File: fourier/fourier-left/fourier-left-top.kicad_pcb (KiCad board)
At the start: 2 copper layers, 136.6 x 96.2 mm, 7 parts

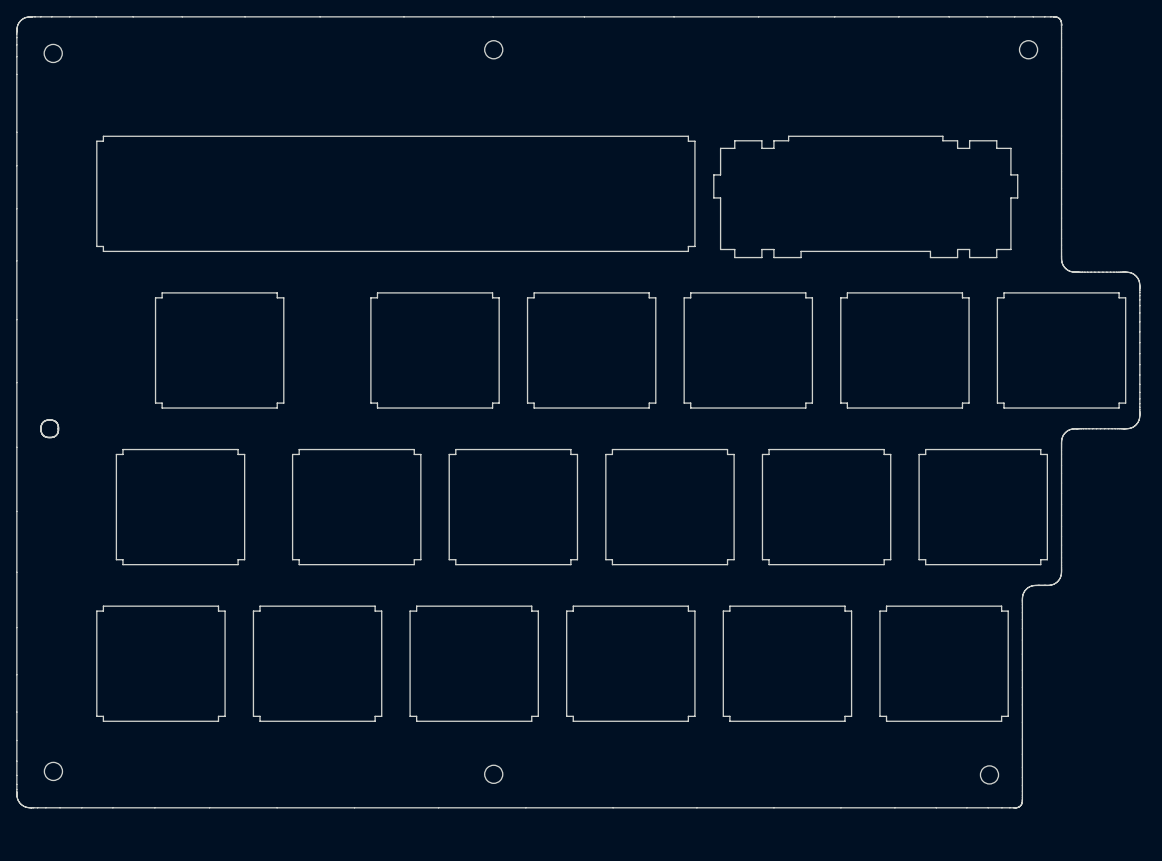
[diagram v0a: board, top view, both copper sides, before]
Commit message: rotate left-top and update to KiCad 5.99
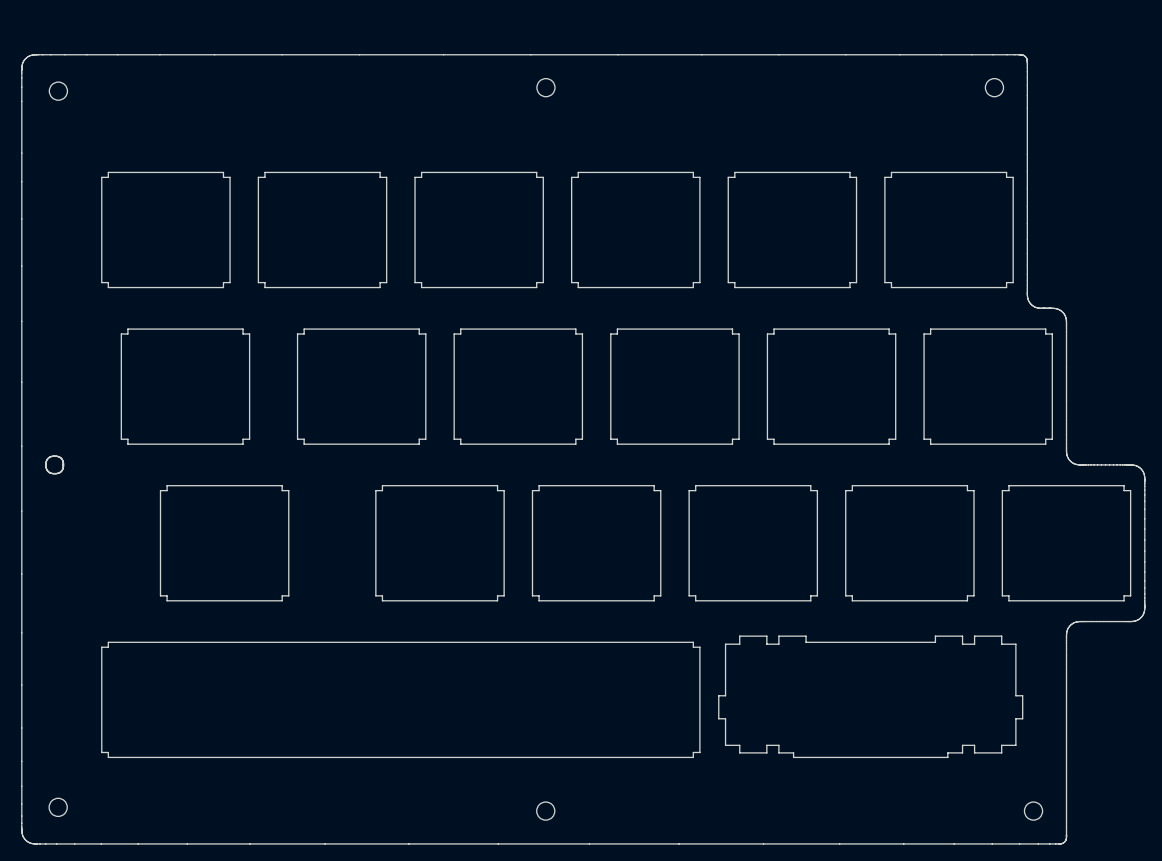
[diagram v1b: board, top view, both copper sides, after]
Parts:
- removed the REF** at (78.0, 111.0)
- removed the REF** at (138.3, 111.1)
- removed the REF** at (143.1, 22.9)
- removed the REF** at (78.0, 22.9)
- removed the REF** at (24.4, 23.3)
- removed the REF** at (24.0, 69.0)
- removed the REF** at (24.4, 110.7)
- added REF**: MountingHole_2.2mm_M2, Mounting_Holes:MountingHole_2.2mm_M2, F.Cu at (138.9, 27.5)
- added REF**: MountingHole_2.2mm_M2, Mounting_Holes:MountingHole_2.2mm_M2, F.Cu at (25.1, 27.9)
- added REF**: MountingHole_2.2mm_M2, Mounting_Holes:MountingHole_2.2mm_M2, F.Cu at (25.0, 115.0)
- added REF**: MountingHole_2.2mm_M2, Mounting_Holes:MountingHole_2.2mm_M2, F.Cu at (24.6, 73.4)
- added REF**: MountingHole_2.2mm_M2, Mounting_Holes:MountingHole_2.2mm_M2, F.Cu at (143.7, 115.5)
- added REF**: MountingHole_2.2mm_M2, Mounting_Holes:MountingHole_2.2mm_M2, F.Cu at (84.4, 27.5)
- added REF**: MountingHole_2.2mm_M2, Mounting_Holes:MountingHole_2.2mm_M2, F.Cu at (84.3, 115.5)
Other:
- board size 136.6 x 96.2 mm -> 136.6 x 96 mm
- net class Default removed
